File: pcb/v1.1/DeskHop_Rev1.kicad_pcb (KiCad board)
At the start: 2 copper layers, 66.9 x 74.5 mm, 20 parts, among them J1 Keyboard In, J2 Debug2, J3 Debug1, J4 Mouse In, U2 Pico Primary Custom, U3 TPD4E1U06DBVR, U4 ADuM1201BR, U5 TPD4E1U06DBVR, U6 Pico Primary Custom

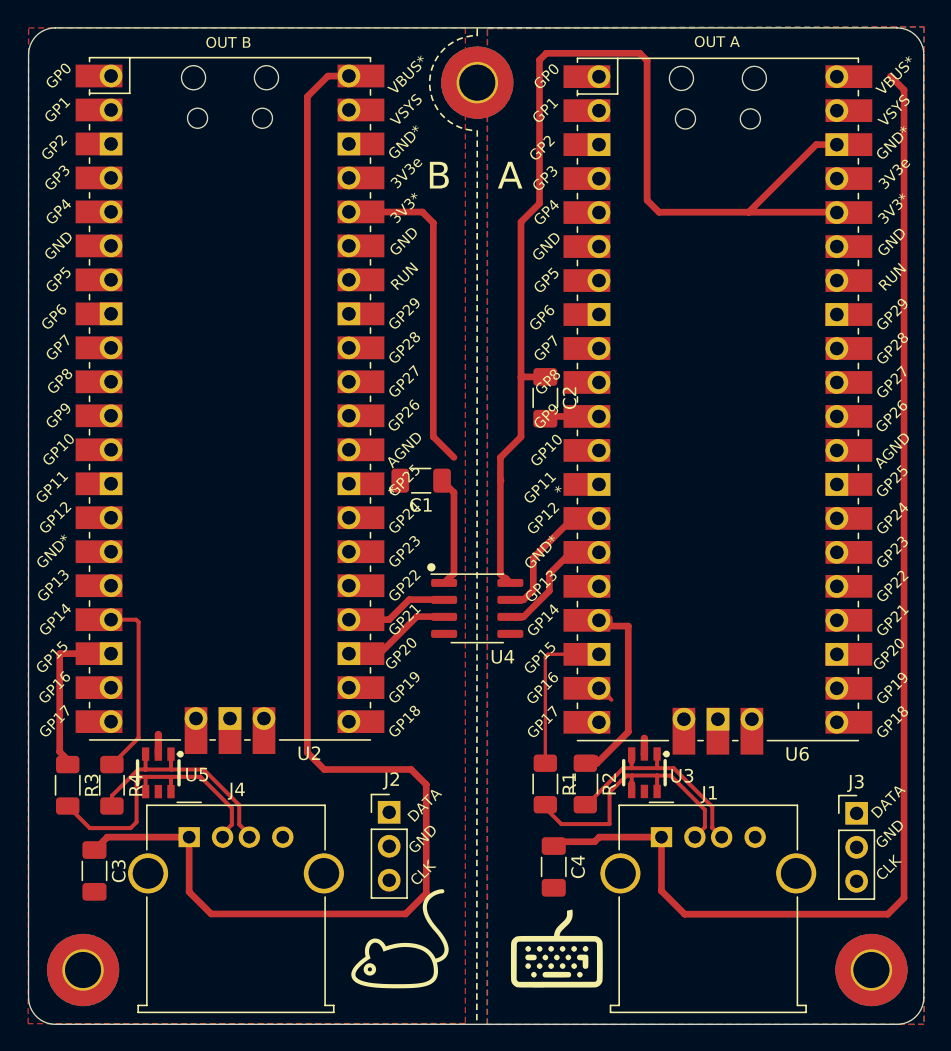
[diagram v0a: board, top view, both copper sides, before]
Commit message: somewhat verOneZeroOne
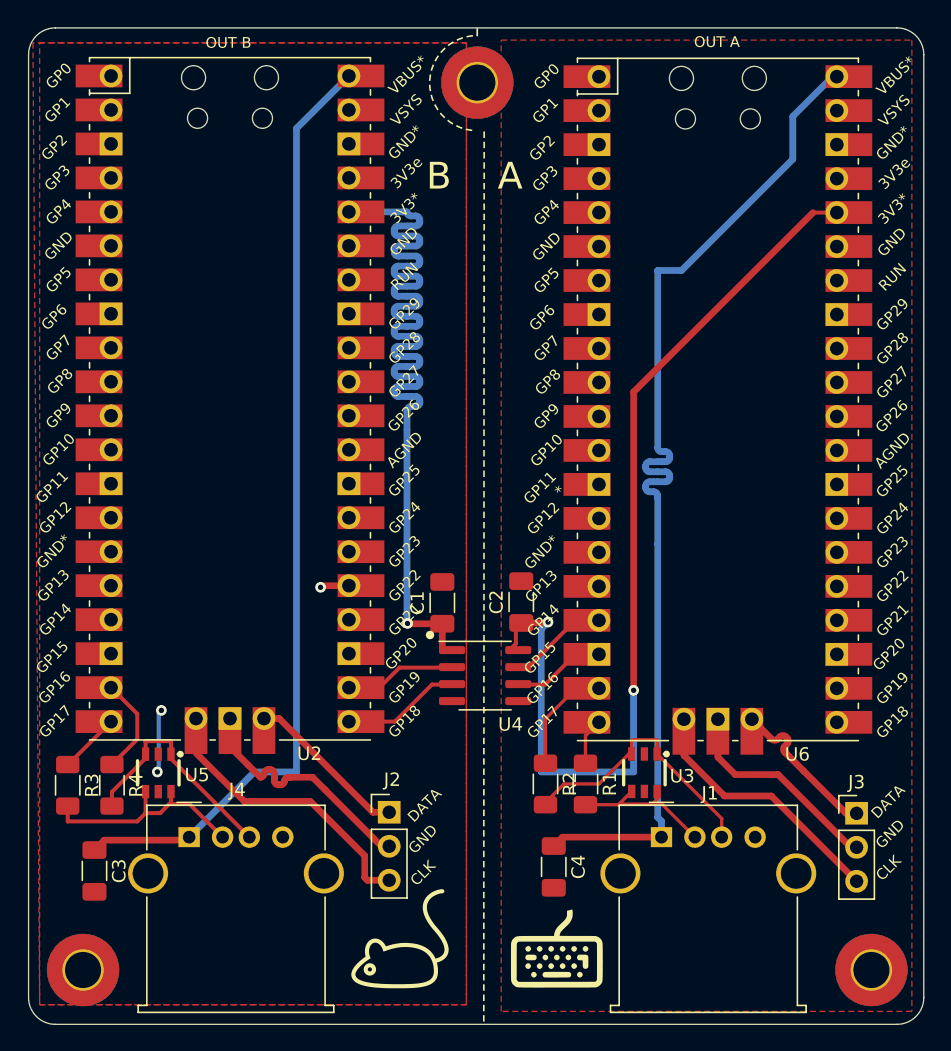
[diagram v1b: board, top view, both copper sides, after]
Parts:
- moved C2 15.4 mm to (70.6, 84.0), turned to 90 degrees
- moved C1 9.27 mm to (64.7, 84.1), turned to 90 degrees
- moved U4 5.06 mm to (67.9, 89.5)
- moved R1 3.00 mm to (75.4, 97.6)
- moved R2 2.98 mm to (72.4, 97.6)
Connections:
- C1 pad 1: 3V3_BUS2 -> 3V3
- C1 pad 2: GND -> GND1
- C3 pad 2: GND -> GND1
- J2 pad 1: unconnected-(J2-Pin_1-Pad1) -> Net-(J2-Pin_1)
- J2 pad 2: GND -> Net-(J2-Pin_2)
- J2 pad 3: unconnected-(J2-Pin_3-Pad3) -> Net-(J2-Pin_3)
- J3 pad 1: unconnected-(J3-Pin_1-Pad1) -> Net-(J3-Pin_1)
- J3 pad 2: GND2 -> Net-(J3-Pin_2)
- J3 pad 3: unconnected-(J3-Pin_3-Pad3) -> Net-(J3-Pin_3)
- J4 pad 4: GND -> GND1
- J4 pad 5: GND -> GND1
- R3 pad 1: Net-(U2-GPIO15) -> Net-(U2-GPIO17)
- R4 pad 1: Net-(U2-GPIO14) -> Net-(U2-GPIO16)
- U2 pad 1: GND -> unconnected-(U2-GPIO0-Pad1)
- U2 pad 11: GND -> unconnected-(U2-GPIO9-Pad11)
- U2 pad 15: unconnected-(U2-GND-Pad15) -> GND1
- U2 pad 16: GND -> unconnected-(U2-GPIO13-Pad16)
- U2 pad 17: Net-(U2-GPIO14) -> unconnected-(U2-GPIO14-Pad17)
- U2 pad 18: Net-(U2-GPIO15) -> unconnected-(U2-GPIO15-Pad18)
- U2 pad 19: unconnected-(U2-GPIO16-Pad19) -> Net-(U2-GPIO16)
- U2 pad 20: unconnected-(U2-GPIO17-Pad20) -> Net-(U2-GPIO17)
- U2 pad 21: unconnected-(U2-GPIO18-Pad21) -> UART B TX
- U2 pad 22: unconnected-(U2-GPIO19-Pad22) -> UART B RX
- U2 pad 23: UART B TX -> unconnected-(U2-GPIO20-Pad23)
- U2 pad 24: UART B RX -> unconnected-(U2-GPIO21-Pad24)
- U2 pad 25: GND -> unconnected-(U2-GPIO22-Pad25)
- U2 pad 30: GND -> unconnected-(U2-GPIO26-Pad30)
- U2 pad 36: unconnected-(U2-3V3-Pad36) -> 3V3
- U2 pad 38: 3V3_BUS2 -> unconnected-(U2-GND-Pad38)
- U2 pad 40: GND -> VBUS2
- U2 pad 41: unconnected-(U2-SWCLK-Pad41) -> Net-(J2-Pin_3)
- U2 pad 42: unconnected-(U2-GND-Pad42) -> Net-(J2-Pin_2)
- U2 pad 43: unconnected-(U2-SWDIO-Pad43) -> Net-(J2-Pin_1)
- U2 pad 6: GND -> GND1
- U4 pad 1: 3V3_BUS2 -> 3V3
- U4 pad 4: GND -> GND1
- U5 pad 2: GND -> GND1
- U6 pad 1: GND2 -> unconnected-(U6-GPIO0-Pad1)
- U6 pad 11: GND2 -> unconnected-(U6-GPIO9-Pad11)
- U6 pad 14: UART A TX -> unconnected-(U6-GPIO12-Pad14)
- U6 pad 15: UART A RX -> GND2
- U6 pad 16: GND2 -> unconnected-(U6-GPIO13-Pad16)
- U6 pad 17: /AD+ -> UART A TX
- U6 pad 18: /AD- -> UART A RX
- U6 pad 19: unconnected-(U6-GPIO16-Pad19) -> /AD+
- U6 pad 2: GND2 -> unconnected-(U6-GPIO1-Pad2)
- U6 pad 20: unconnected-(U6-GPIO17-Pad20) -> /AD-
- U6 pad 21: GND2 -> unconnected-(U6-GPIO18-Pad21)
- U6 pad 25: GND2 -> unconnected-(U6-GPIO22-Pad25)
- U6 pad 30: GND2 -> unconnected-(U6-GPIO26-Pad30)
- U6 pad 35: unconnected-(U6-GND-Pad35) -> GND2
- U6 pad 36: unconnected-(U6-3V3-Pad36) -> Net-(U4-VDD2)
- U6 pad 38: Net-(U4-VDD2) -> GND2
- U6 pad 40: GND2 -> VBUS1
- U6 pad 41: unconnected-(U6-SWCLK-Pad41) -> Net-(J3-Pin_3)
- U6 pad 42: unconnected-(U6-GND-Pad42) -> Net-(J3-Pin_2)
- U6 pad 43: unconnected-(U6-SWDIO-Pad43) -> Net-(J3-Pin_1)
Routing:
- net 3V3: track 0.00 -> 70.6 mm, vias 0 -> 1
- net VBUS2: track 101.4 -> 71.2 mm
- net unconnected-(U2-3V3-Pad36): track 24.8 -> 0.00 mm
- net Net-(J3-Pin_3): track 0.00 -> 19.5 mm
- net Net-(J2-Pin_3): track 0.00 -> 19.3 mm
- net Net-(J3-Pin_2): track 0.00 -> 18.4 mm
- net Net-(J2-Pin_2): track 0.00 -> 16.4 mm
- net VBUS1: track 93.5 -> 77.8 mm
- net Net-(U2-GPIO14): track 13.8 -> 0.00 mm
- net Net-(U4-VDD2): track 85.2 -> 71.9 mm, vias 0 -> 2
- net Net-(U2-GPIO15): track 12.5 -> 0.00 mm
- net Net-(J2-Pin_1): track 0.00 -> 12.3 mm
- net Net-(J3-Pin_1): track 0.00 -> 12.2 mm
- net OA-: track 22.0 -> 11.7 mm
- net 3V3_BUS2: track 8.82 -> 0.00 mm
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- added copper zone on F.Cu, net GND1
- added copper zone on F.Cu, net unconnected-(U2-GPIO22-Pad25)
- removed copper zone on F.Cu, net GND
- removed copper zone on B.Cu, net GND2
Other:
- board text added: "GND*"
- board text removed: "${REFERENCE}"

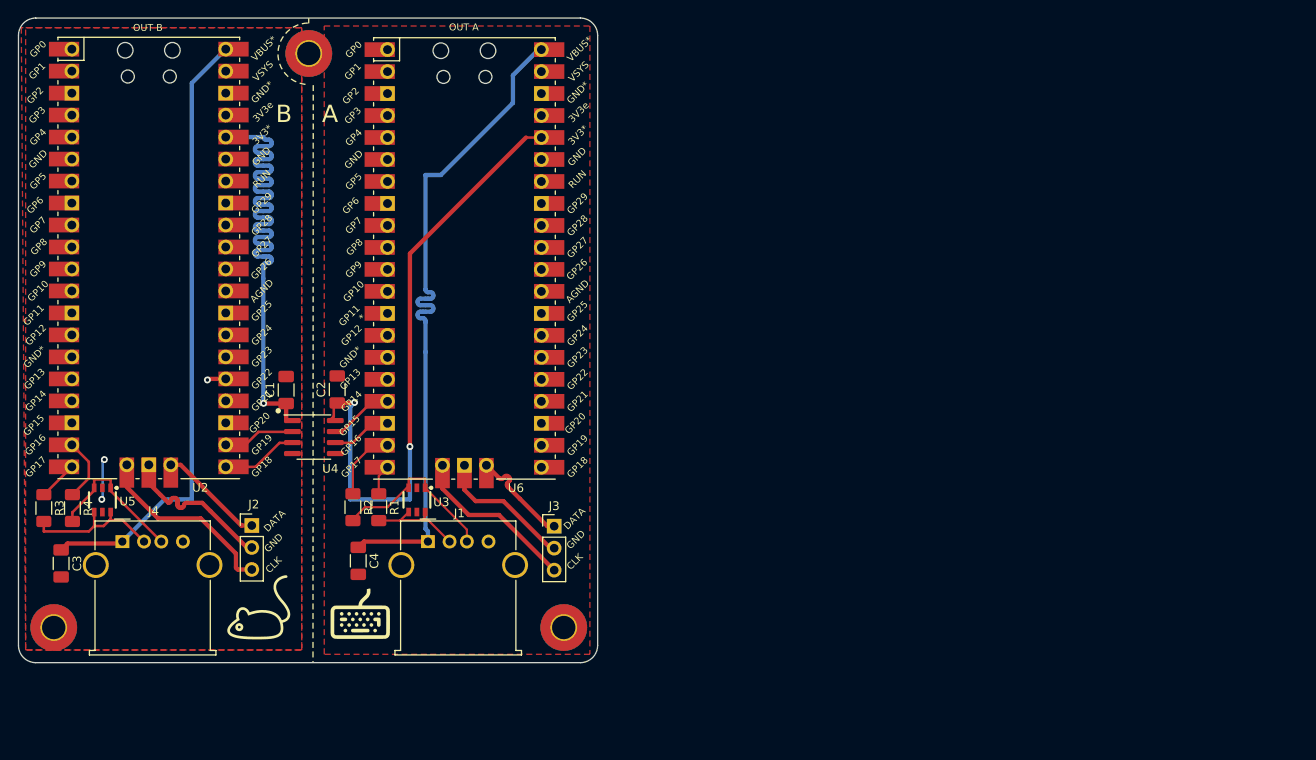
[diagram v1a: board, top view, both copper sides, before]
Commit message: ver OneXeroOne
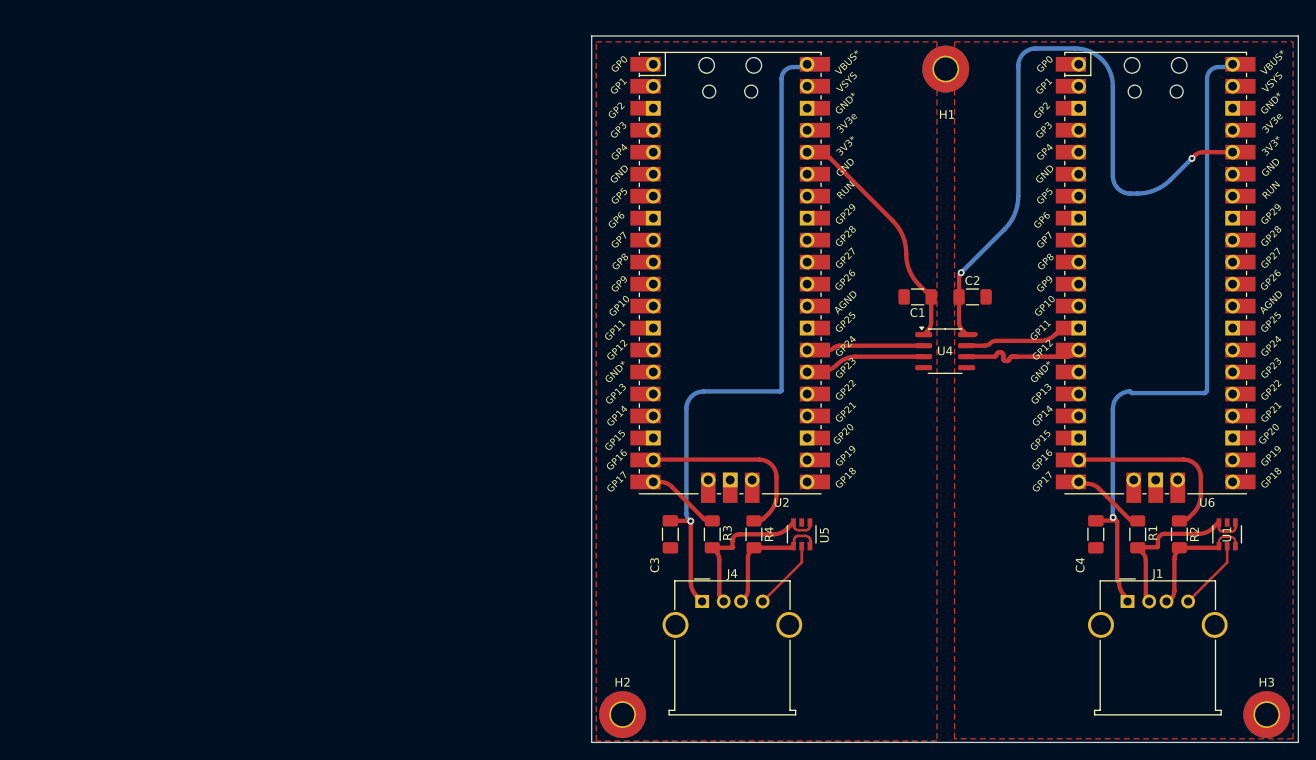
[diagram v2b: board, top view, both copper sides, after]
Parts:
- removed J2: Debug2, Connector_PinHeader_2.54mm:PinHeader_1x03_P2.54mm_Vertical
- removed J3: Debug1, Connector_PinHeader_2.54mm:PinHeader_1x03_P2.54mm_Vertical
- removed U3: TPD4E1U06DBVR, Library:TPD4E1U06DBVR
- added U1: TPD4E1U06DBVR, Customs:DBV6_TEX, F.Cu at (173.4, 100.7)
- U5: footprint Library:TPD4E1U06DBVR -> Customs:DBV6_TEX
- moved H3 134.5 mm to (178.0, 121.6)
- moved H1 121.6 mm to (140.9, 47.0)
- moved R2 95.5 mm to (167.9, 100.7)
- moved R1 87.7 mm to (163.1, 100.7)
- moved C4 85.3 mm to (158.3, 100.7)
- moved J1 81.1 mm to (161.9, 108.5)
- moved U5 80.9 mm to (124.3, 100.7)
- moved U6 79.9 mm to (165.2, 70.6)
- moved R4 78.8 mm to (118.7, 100.7)
- moved R3 77.3 mm to (113.9, 100.7)
- moved C2 74.2 mm to (144.0, 73.3), turned to 0 degrees
- moved C1 73.8 mm to (137.7, 73.3), turned to 180 degrees
- moved U4 73.6 mm to (140.8, 79.6)
- moved C3 70.5 mm to (109.1, 100.7)
- moved J4 67.3 mm to (112.8, 108.5)
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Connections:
- H1 pad 1: GND -> GND2
- H2 pad 1: GND2 -> GND1
- U2 pad 21: UART B TX -> unconnected-(U2-GPIO18-Pad21)
- U2 pad 22: UART B RX -> unconnected-(U2-GPIO19-Pad22)
- U2 pad 26: unconnected-(U2-GPIO23-Pad26) -> UART B TX
- U2 pad 27: unconnected-(U2-GPIO24-Pad27) -> UART B RX
- U2 pad 41: Net-(J2-Pin_3) -> unconnected-(U2-SWCLK-Pad41)
- U2 pad 42: Net-(J2-Pin_2) -> unconnected-(U2-GND-Pad42)
- U2 pad 43: Net-(J2-Pin_1) -> unconnected-(U2-SWDIO-Pad43)
- U6 pad 13: unconnected-(U6-GPIO11-Pad13) -> UART A TX
- U6 pad 14: unconnected-(U6-GPIO12-Pad14) -> UART A RX
- U6 pad 17: UART A TX -> unconnected-(U6-GPIO14-Pad17)
- U6 pad 18: UART A RX -> unconnected-(U6-GPIO15-Pad18)
- U6 pad 41: Net-(J3-Pin_3) -> unconnected-(U6-SWCLK-Pad41)
- U6 pad 42: Net-(J3-Pin_2) -> unconnected-(U6-GND-Pad42)
- U6 pad 43: Net-(J3-Pin_1) -> unconnected-(U6-SWDIO-Pad43)
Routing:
- net 3V3: track 70.6 -> 27.8 mm, vias 1 -> 0
- net Net-(J3-Pin_3): track 19.5 -> 0.00 mm
- net Net-(J2-Pin_3): track 19.3 -> 0.00 mm
- net Net-(J3-Pin_2): track 18.4 -> 0.00 mm
- net Net-(J2-Pin_2): track 16.4 -> 0.00 mm
- net Net-(U2-GPIO16): track 7.35 -> 21.8 mm
- net /AD+: track 8.26 -> 21.7 mm
- net Net-(J2-Pin_1): track 12.3 -> 0.00 mm
- net Net-(J3-Pin_1): track 12.2 -> 0.00 mm
- net OA-: track 11.7 -> 20.8 mm
- net GND2: track 0.00 -> 8.26 mm
- net UART A RX: track 7.66 -> 14.5 mm
- net OA+: track 20.3 -> 13.8 mm
- net VBUS2: track 71.2 -> 77.2 mm, vias 0 -> 1
- net UART B RX: track 7.64 -> 13.6 mm
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- removed copper zone on F.Cu, net unconnected-(U2-GPIO22-Pad25)
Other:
- board size 66.9 x 74.5 mm -> 81.7 x 81.6 mm
- board text removed: "*"
- board text removed: "A"
- board text removed: "B"
- board text removed: "CLK"
- board text removed: "DATA"
- board text removed: "DeskHop"
- board text removed: "GND"
- board text removed: "GND*"
- board text removed: "Keyboard/Mouse Switch"
- board text removed: "OUT A"
- board text removed: "OUT B"
- board text removed: "by Hrvoje Cavrak, 01/24"
- board text removed: "https://github.com/hrvach"
- board text removed: "rev 1.1"
